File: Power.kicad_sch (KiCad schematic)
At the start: 90 parts, among them U1 TPS546D24ARVFR, U4 TPS546D24ARVFR, U5 RT9080-33GJ5, U7 LMR54410

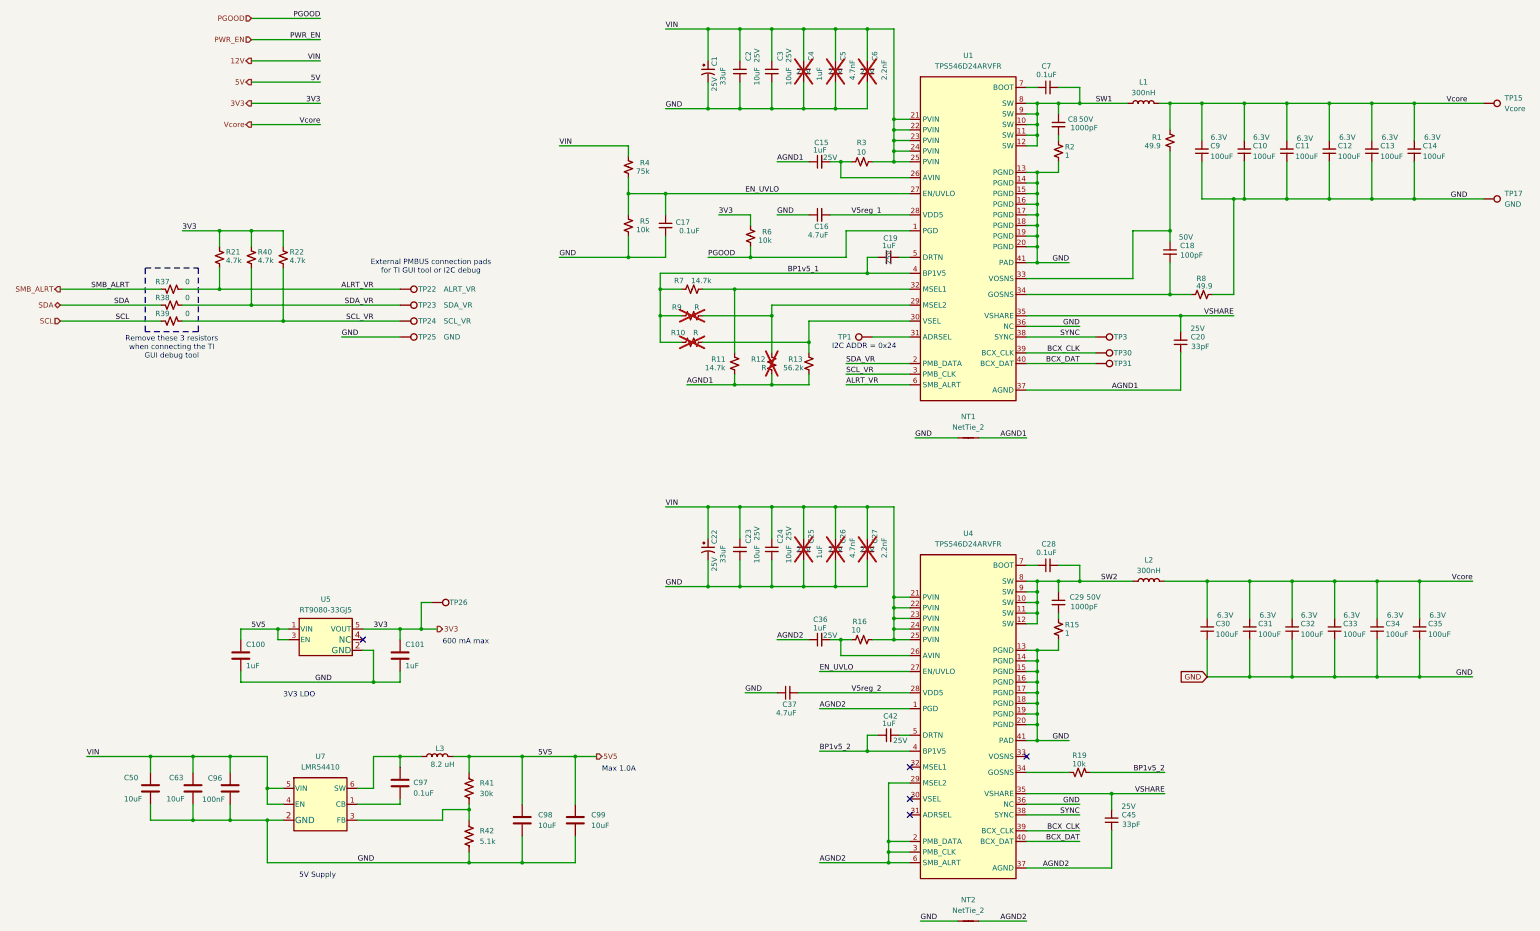
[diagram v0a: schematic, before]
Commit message: final update
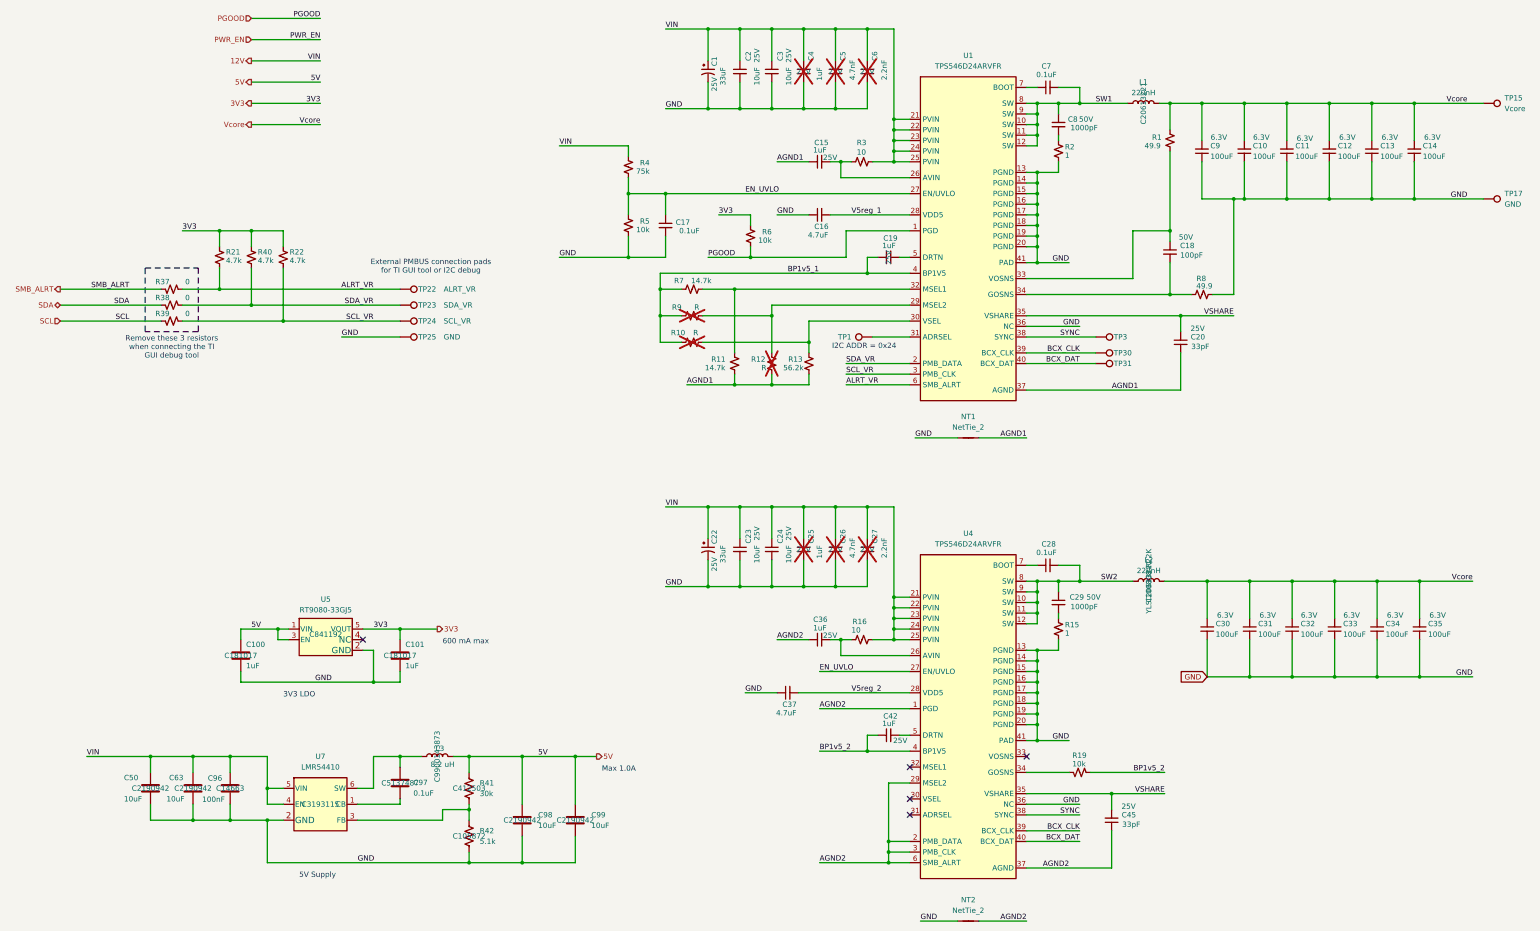
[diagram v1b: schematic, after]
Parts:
- removed TP26: TestPoint, TestPoint:TestPoint_Pad_D1.0mm, symbol Connector:TestPoint
- C100, C101: LCSC (none) -> C181017
- C50, C63, C98, C99: LCSC (none) -> C2190942
- C96: LCSC (none) -> C14663
- C97: LCSC (none) -> C5137487
- L1, L2: value 300nH -> 220nH; DK (none) -> YLSI100808-R22K; LCSC (none) -> C20613221; PARTNO SLC1175-271MEC -> YLSI100808-R22K
- L3: LCSC (none) -> C9900143873
- R41: LCSC (none) -> C412503
- R42: LCSC (none) -> C105872
- U5: LCSC (none) -> C841192
- U7: LCSC (none) -> C3193115
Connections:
- net 5V5 is gone; now on net 5V: C100.1, C98.1, C99.1, L3.2, R41.1, U5.1 (VIN), U5.3 (EN)
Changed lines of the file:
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@@
 	)
 	(junction
-		(at 124.46 180.34)
-		(diameter 0)
-		(color 0 0 0 0)
-	)
-	(junction
 		(at 181.61 105.41)
 		(diameter 0)
@@
 	(wire
 		(pts
-			(xy 124.46 180.34) (xy 128.27 180.34)
+			(xy 119.38 180.34) (xy 128.27 180.34)
 		)
 		(stroke
@@
 	(wire
 		(pts
-			(xy 127 173.99) (xy 124.46 173.99)
-		)
-		(stroke
-			(width 0)
-			(type default)
-		)
-	)
-	(wire
-		(pts
 			(xy 200.66 163.83) (xy 200.66 170.18)
 		)
@@
 	(wire
 		(pts
-			(xy 124.46 173.99) (xy 124.46 180.34)
-		)
-		(stroke
-			(width 0)
-			(type default)
-		)
-	)
-	(wire
-		(pts
 			(xy 237.49 66.04) (xy 241.3 66.04)
 		)
@@
 	(wire
 		(pts
-			(xy 119.38 180.34) (xy 124.46 180.34)
-		)
-		(stroke
-			(width 0)
-			(type default)
-		)
-	)
-	(wire
-		(pts
 			(xy 269.24 168.91) (xy 271.78 168.91)
 		)
@@
 		)
 	)
-	(label "5V5"
+	(label "5V"
 		(at 152.4 210.82 0)
 		(effects
@@
 		)
 	)
-	(label "5V5"
+	(label "5V"
 		(at 83.82 180.34 0)
 		(effects
@@
 		)
 	)
-	(hierarchical_label "5V5"
+	(hierarchical_label "5V"
 		(shape output)
 		(at 166.37 210.82 0)
@@
 			)
 		)
+		(property "LCSC" "C14663"
+			(at 78.74 218.44 0)
+			(effects
+				(font
+					(size 1.27 1.27)
+				)
+			)
+		)
 		(pin "1"
 		)
@@
 			)
 		)
+		(property "LCSC" "C2190942"
+			(at 161.29 226.06 0)
+			(effects
+				(font
+					(size 1.27 1.27)
+				)
+			)
+		)
 		(pin "1"
 		)
@@
 			)
 		)
+		(property "LCSC" "C5137487"
+			(at 119.38 217.17 0)
+			(effects
+				(font
+					(size 1.27 1.27)
+				)
+			)
+		)
 		(pin "1"
 		)
@@
 			)
 		)
+		(property "LCSC" "C2190942"
+			(at 148.59 226.06 0)
+			(effects
+				(font
+					(size 1.27 1.27)
+				)
+			)
+		)
 		(pin "1"
 		)
@@
 			)
 		)
+		(property "LCSC" "C181017"
+			(at 81.28 186.69 0)
+			(effects
+				(font
+					(size 1.27 1.27)
+				)
+			)
+		)
 		(pin "1"
 		)
@@
 			)
 		)
-		(property "Value" "300nH"
+		(property "Value" "220nH"
 			(at 297.18 52.07 90)
 			(effects
@@
 			)
 		)
-		(property "PARTNO" "SLC1175-271MEC"
+		(property "PARTNO" "YLSI100808-R22K"
 			(at 297.18 54.61 90)
 			(effects
@@
 			)
 		)
-		(property "DK" ""
+		(property "DK" "YLSI100808-R22K"
 			(at 297.18 54.61 0)
 			(effects
@@
 			)
 		)
+		(property "LCSC" "C20613221"
+			(at 297.18 54.61 0)
+			(effects
+				(font
+					(size 1.27 1.27)
+				)
+			)
+		)
 		(pin "1"
 		)
@@
 			)
 		)
+		(property "LCSC" "C841192"
+			(at 101.6 181.61 0)
+			(effects
+				(font
+					(size 1.27 1.27)
+				)
+			)
+		)
 		(pin "1"
 		)
@@
 			)
 		)
+		(property "LCSC" "C3193115"
+			(at 100.33 222.25 0)
+			(effects
+				(font
+					(size 1.27 1.27)
+				)
+			)
+		)
 		(pin "1"
 		)
@@
 	)
 	(symbol
-		(lib_id "Connector:TestPoint")
-		(at 127 173.99 270)
-		(mirror x)
-		(unit 1)
-		(exclude_from_sim no)
-		(in_bom no)
-		(on_board yes)
-		(dnp no)
-		(property "Reference" "TP26"
-			(at 133.35 173.99 90)
-			(effects
-				(font
-					(size 1.27 1.27)
-				)
-			)
-		)
-		(property "Value" "TestPoint"
-			(at 132.715 172.7201 90)
-			(effects
-				(font
-					(size 1.27 1.27)
-				)
-				(justify left)
-				(hide yes)
-			)
-		)
-		(property "Footprint" "TestPoint:TestPoint_Pad_D1.0mm"
-			(at 127 168.91 0)
-			(effects
-				(font
-					(size 1.27 1.27)
-				)
-				(hide yes)
-			)
-		)
-		(property "Datasheet" "~"
-			(at 127 168.91 0)
-			(effects
-				(font
-					(size 1.27 1.27)
-				)
-				(hide yes)
-			)
-		)
-		(property "Description" ""
-			(at 127 173.99 0)
-			(effects
-				(font
-					(size 1.27 1.27)
-				)
-				(hide yes)
-			)
-		)
-		(property "嘉立创元件编号" ""
-			(at 127 173.99 0)
-			(effects
-				(font
-					(size 1.27 1.27)
-				)
-				(hide yes)
-			)
-		)
-		(pin "1"
-		)
-		(instances
-			(project "BitaxeGT"
-				(path "/61fe8d2c-9301-4ad9-8caf-c47acfa835b0/24036843-8461-4d4b-b738-f953c909ed6c"
-					(reference "TP26")
-					(unit 1)
-				)
-			)
-		)
-	)
-	(symbol
 		(lib_id "Device:R_Small_US")
 		(at 229.87 182.88 270)
@@
 			)
 		)
+		(property "LCSC" "C181017"
+			(at 119.38 186.69 0)
+			(effects
+				(font
+					(size 1.27 1.27)
+				)
+			)
+		)
 		(pin "1"
 		)
@@
 			)
 		)
+		(property "LCSC" "C9900143873"
+			(at 128.27 210.82 0)
+			(effects
+				(font
+					(size 1.27 1.27)
+				)
+			)
+		)
 		(pin "1"
 		)
@@
 			)
 		)
+		(property "LCSC" "C105872"
+			(at 135.89 229.87 0)
+			(effects
+				(font
+					(size 1.27 1.27)
+				)
+			)
+		)
 		(pin "1"
 		)
@@
 			)
 		)
+		(property "LCSC" "C412503"
+			(at 135.89 218.44 0)
+			(effects
+				(font
+					(size 1.27 1.27)
+				)
+			)
+		)
 		(pin "1"
 		)
@@
 			)
 		)
-		(property "Value" "300nH"
+		(property "Value" "220nH"
 			(at 298.45 166.37 90)
 			(effects
@@
 			)
 		)
-		(property "PARTNO" "SLC1175-271MEC"
+		(property "PARTNO" "YLSI100808-R22K"
 			(at 298.45 168.91 90)
 			(effects
@@
 			)
 		)
-		(property "DK" ""
+		(property "DK" "YLSI100808-R22K"
+			(at 298.45 168.91 0)
+			(effects
+				(font
+					(size 1.27 1.27)
+				)
+			)
+		)
+		(property "LCSC" "C20613221"
 			(at 298.45 168.91 0)
 			(effects
@@
 			)
 		)
+		(property "LCSC" "C2190942"
+			(at 69.85 218.44 0)
+			(effects
+				(font
+					(size 1.27 1.27)
+				)
+			)
+		)
 		(pin "1"
 		)
@@
 			)
 		)
+		(property "LCSC" "C2190942"
+			(at 59.69 218.44 0)
+			(effects
+				(font
+					(size 1.27 1.27)
+				)
+			)
+		)

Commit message: change cap
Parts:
- C15, C19, C36, C42: LCSC C92827 -> C77009
- C16, C37: LCSC C335105 -> C23733
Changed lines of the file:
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@@
 			)
 		)
-		(property "LCSC" "C92827"
+		(property "LCSC" "C77009"
 			(at 236.22 91.44 90)
 			(effects
@@
 			)
 		)
-		(property "LCSC" "C335105"
+		(property "LCSC" "C23733"
 			(at 212.09 195.58 90)
 			(effects
@@
 			)
 		)
-		(property "LCSC" "C92827"
+		(property "LCSC" "C77009"
 			(at 219.71 68.58 90)
 			(effects
@@
 			)
 		)
-		(property "LCSC" "C92827"
+		(property "LCSC" "C77009"
 			(at 219.71 182.88 90)
 			(effects
@@
 			)
 		)
-		(property "LCSC" "C335105"
+		(property "LCSC" "C23733"
 			(at 219.71 81.28 90)
 			(effects
@@
 			)
 		)
-		(property "LCSC" "C92827"
+		(property "LCSC" "C77009"
 			(at 236.22 205.74 90)
 			(effects
